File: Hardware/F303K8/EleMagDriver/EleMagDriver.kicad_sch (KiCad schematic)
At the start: 37 parts, among them IC1 BD9E302EFJ-E2, IC2 TBD62083APG, IC3 TBD62083APG, IC4 TBD62083APG, J1 Jack-DC, J10 RelayD, J11 RelayE, J12 RelayF, J13 RelayG, J14 RelayH, J15 RelayI, J16 RelayJ, J17 Floppy_Power, J18 FloppyA, J19 Floppy_Power, J2 MotorDriverIn, J20 FloppyB, J21 Floppy_Power, J22 FloppyC, J3 MotorDriveOut, J4 SolenoidA, J5 SolenoidB, J6 StpMotor, J7 RelayA, J8 RelayB, J9 RelayC, U1 NUCLEO-F303K8

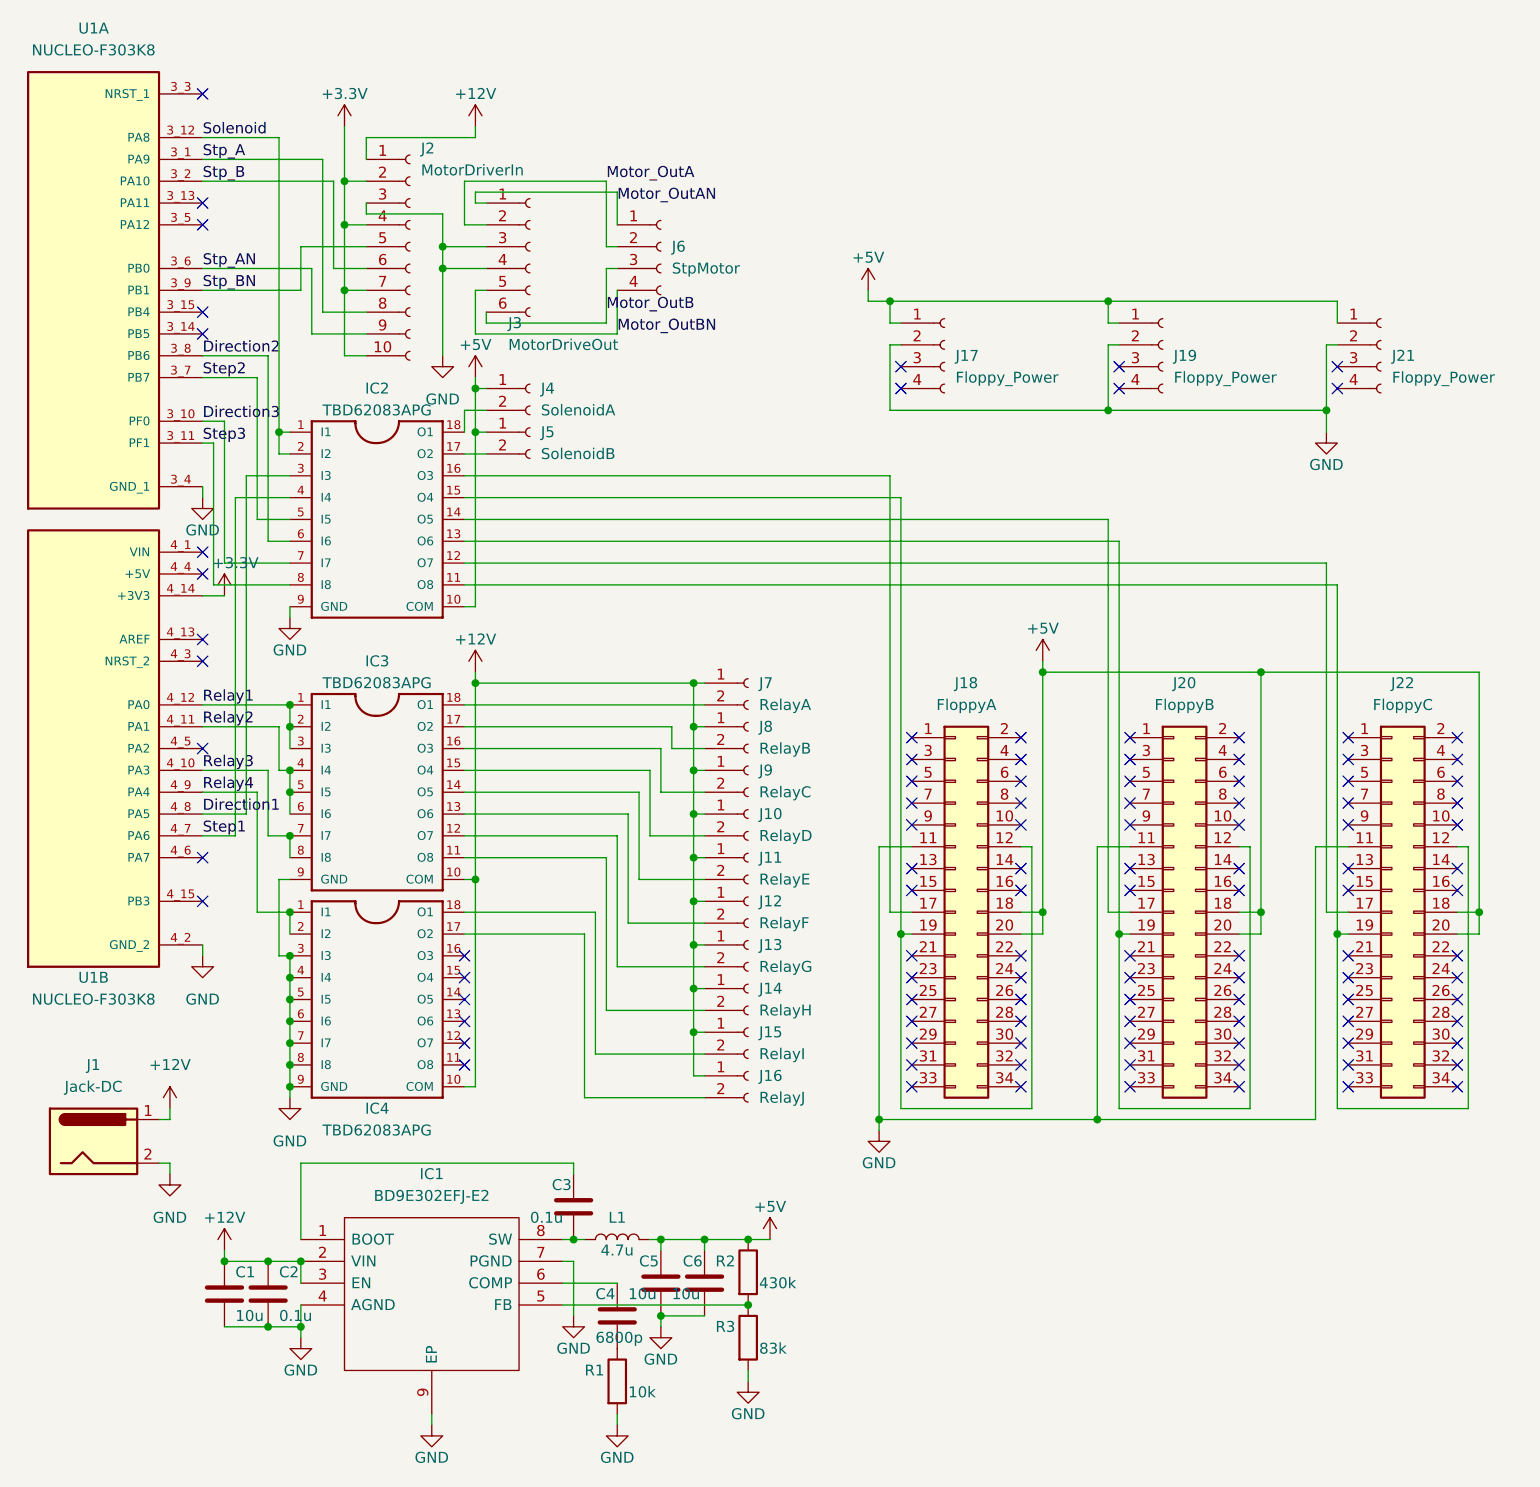
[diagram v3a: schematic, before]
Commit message: edit circuit
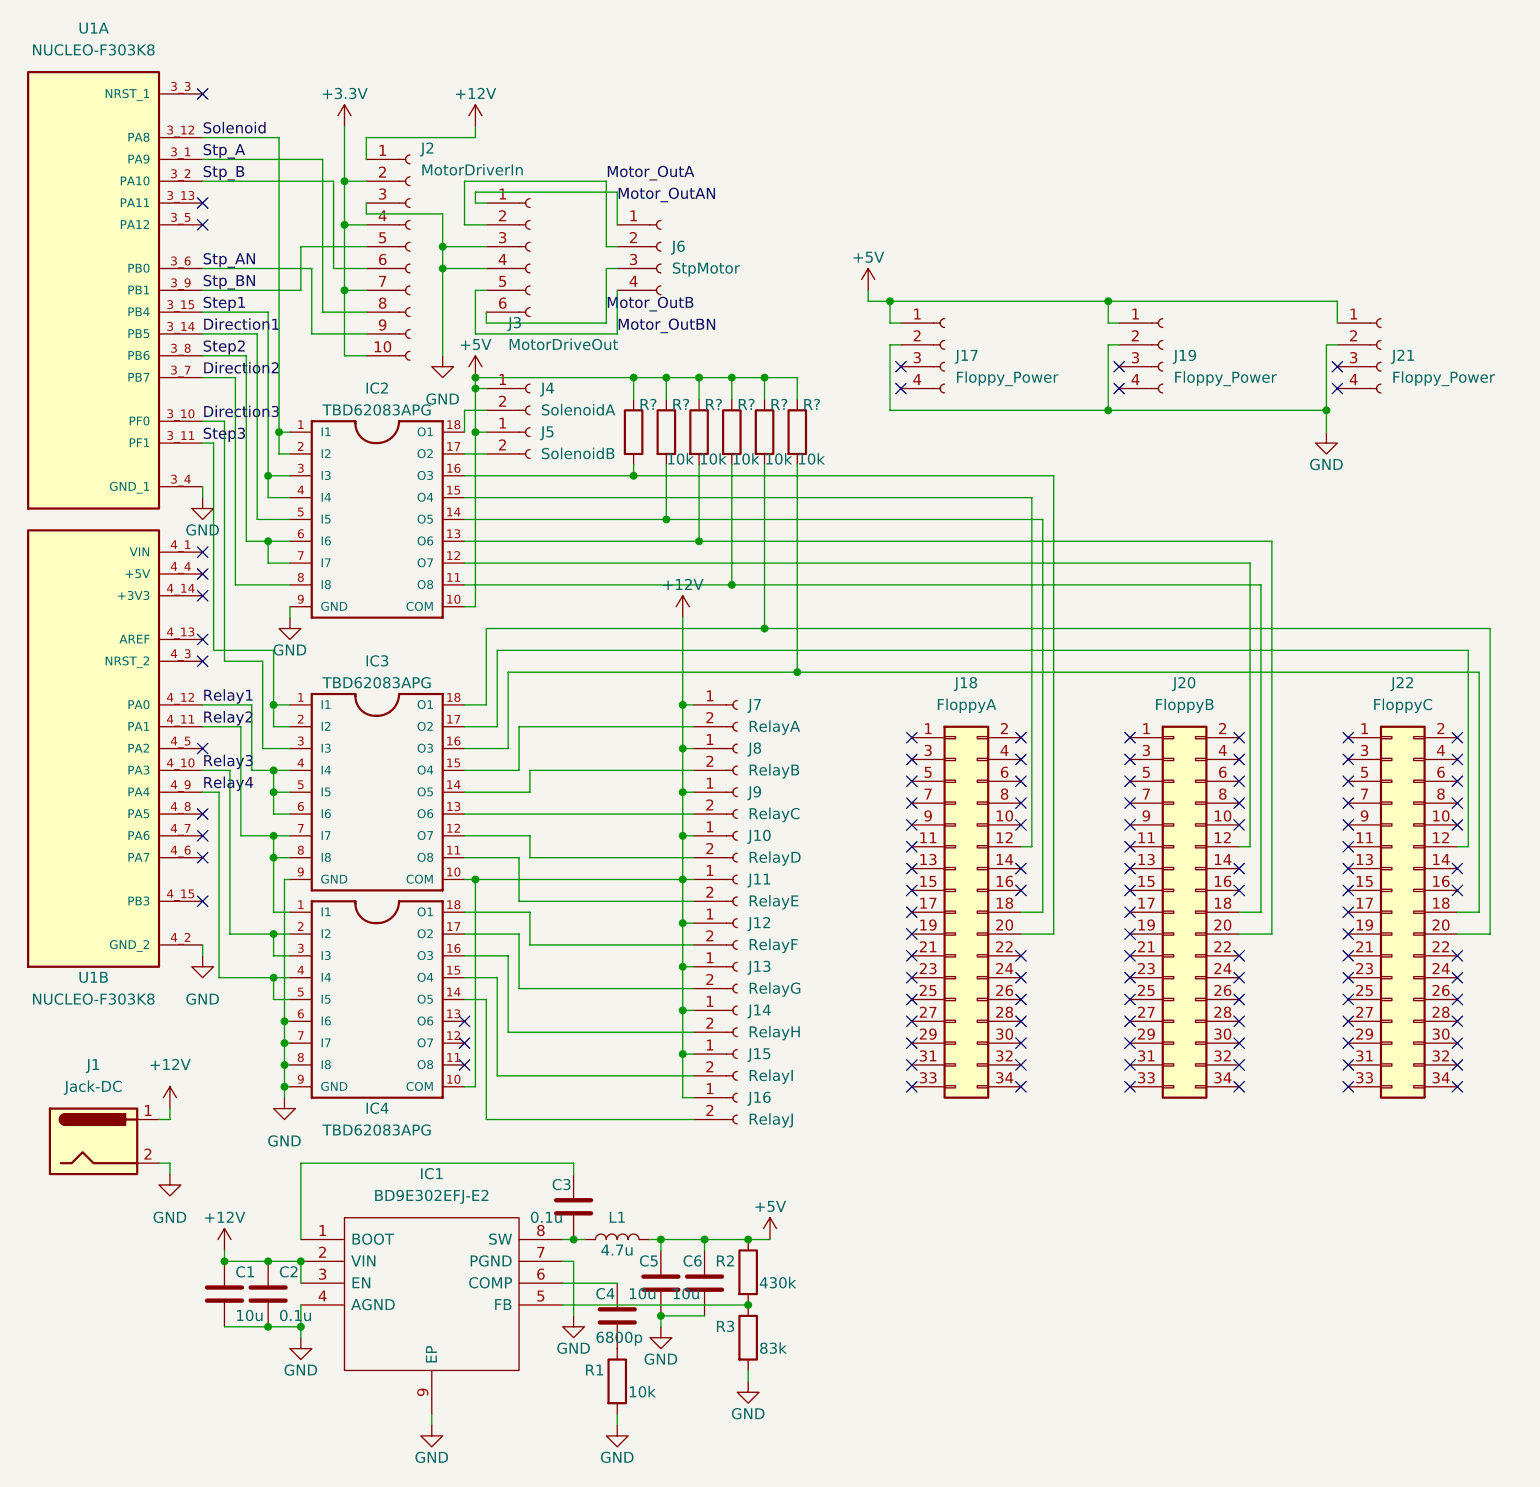
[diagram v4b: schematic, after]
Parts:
- added R? (x5): 10k, symbol Device:R
- added R?: (no value), symbol Device:R
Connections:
- net +3.3V: no longer U1.4_14 (+3V3)
- net +5V: now also R?.1, R?.1, R?.1, R?.1, R?.1, R?.1; no longer J18.18 (Pin_18), J18.20 (Pin_20), J20.18 (Pin_18), J20.20 (Pin_20), J22.18 (Pin_18), J22.20 (Pin_20)
- net Direction1: now also IC2.5 (I5), U1.3_14 (PB5); no longer IC2.3 (I3), U1.4_8 (PA5)
- net Direction2: now also IC2.8 (I8), U1.3_7 (PB7); no longer IC2.6 (I6), U1.3_8 (PB6)
- net Direction3: now also IC3.3 (I3); no longer IC2.7 (I7)
- net GND: no longer IC4.3 (I3), IC4.4 (I4), IC4.5 (I5), J18.11 (Pin_11), J20.11 (Pin_11), J22.11 (Pin_11)
- net Relay1: now also IC3.4 (I4), IC3.5 (I5), IC3.6 (I6); no longer IC3.1 (I1), IC3.2 (I2), IC3.3 (I3)
- net Relay2: now also IC3.7 (I7), IC3.8 (I8), IC4.1 (I1); no longer IC3.4 (I4), IC3.5 (I5), IC3.6 (I6)
- net Relay3: now also IC4.2 (I2), IC4.3 (I3); no longer IC3.7 (I7), IC3.8 (I8)
- net Relay4: now also IC4.4 (I4), IC4.5 (I5); no longer IC4.1 (I1), IC4.2 (I2)
- net Step1: now also IC2.3 (I3), U1.3_15 (PB4); no longer U1.4_7 (PA6)
- net Step2: now also IC2.6 (I6), IC2.7 (I7), U1.3_8 (PB6); no longer IC2.5 (I5), U1.3_7 (PB7)
- net Step3: now also IC3.1 (I1), IC3.2 (I2); no longer IC2.8 (I8)
- net at J7.2 (Pin_2): now also IC3.15 (O4); no longer IC3.18 (O1)
- net at J10.2 (Pin_2): now also IC3.12 (O7); no longer IC3.15 (O4)
- net at J8.2 (Pin_2): now also IC3.14 (O5); no longer IC3.17 (O2)
- net at IC2.12 (O7): now also J20.12 (Pin_12); no longer J22.17 (Pin_17)
- net at IC2.14 (O5): now also J18.18 (Pin_18), R?.2; no longer J20.17 (Pin_17)
- net at IC2.15 (O4), J18.12 (Pin_12): no longer J18.19 (Pin_19)
- net at IC2.16 (O3): now also J18.20 (Pin_20), R?.2; no longer J18.17 (Pin_17)
- net at J14.2 (Pin_2): now also IC4.16 (O3); no longer IC3.11 (O8)
- net at J11.2 (Pin_2): now also IC3.11 (O8); no longer IC3.14 (O5)
- net at IC4.14 (O5): now also J16.2 (Pin_2)
- net at IC4.15 (O4): now also J15.2 (Pin_2)
- net at IC4.17 (O2): now also J13.2 (Pin_2); no longer J16.2 (Pin_2)
- net at IC4.18 (O1): now also J12.2 (Pin_2); no longer J15.2 (Pin_2)
- net at IC3.13 (O6): now also J9.2 (Pin_2); no longer J12.2 (Pin_2)
- net at IC3.16 (O3): now also J22.18 (Pin_18), R?.2; no longer J9.2 (Pin_2)
- new net: IC2.11 (O8), J20.18 (Pin_18), R?.2
- new net: IC2.13 (O6), J20.20 (Pin_20), R?.2
- new net: IC3.18 (O1), J22.20 (Pin_20), R?.2
- new net: IC3.17 (O2), J22.12 (Pin_12)
- now unconnected: J20.19 (Pin_19), J22.19 (Pin_19)
- no-connect marks 108 -> 115
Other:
- moved on the sheet: J10, J11, J12, J13, J14, J15, J16, J7, J8, J9
